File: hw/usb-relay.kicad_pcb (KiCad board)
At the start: 2 copper layers, 22 parts, among them IC1 ATTINY85-P, K1 RELAY_2RT, P1 USB_B, P2 CONN_02X03, Q1 BC548, U1 LM741

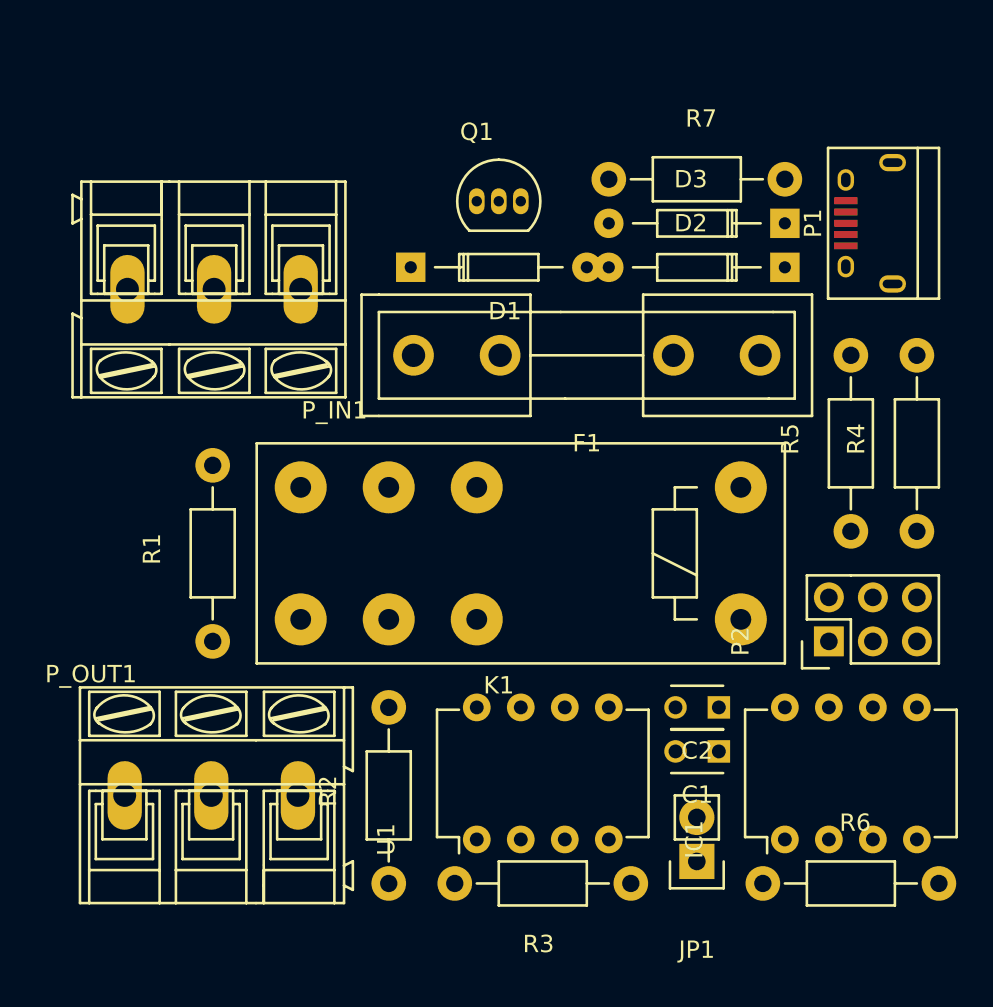
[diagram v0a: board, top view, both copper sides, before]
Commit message: Changes
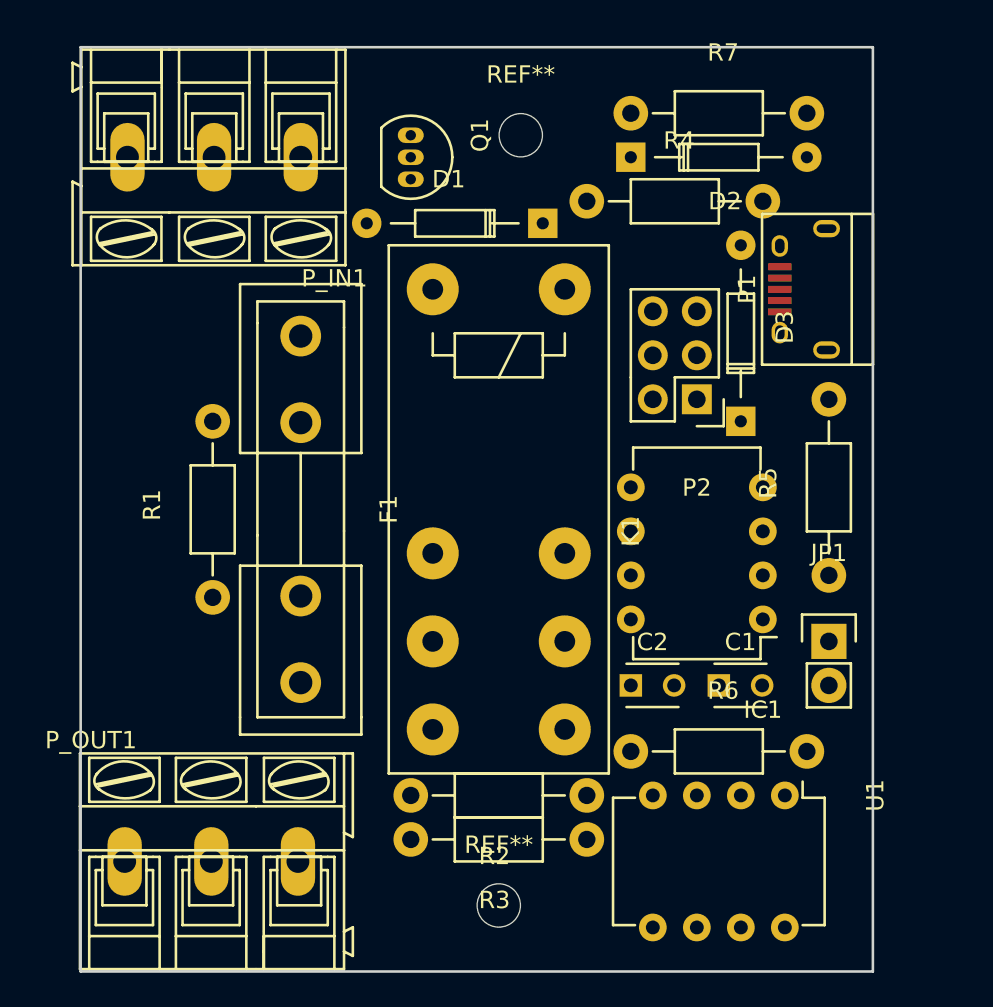
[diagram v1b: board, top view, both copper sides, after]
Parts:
- added REF**: MountingHole_2-5mm, Mounting_Holes:MountingHole_2-5mm, F.Cu at (76.2, 92.7)
- added REF**: MountingHole_2-5mm, Mounting_Holes:MountingHole_2-5mm, F.Cu at (74.9, 137.2)
- moved R4 26.9 mm to (80.0, 96.5), turned to 0 degrees
- moved K1 21.1 mm to (71.1, 101.6), turned to 270 degrees
- moved F1 18.8 mm to (63.5, 114.3), turned to 270 degrees
- moved U1 18.0 mm to (91.4, 130.8), turned to 270 degrees
- moved P2 15.9 mm to (86.4, 108.0), turned to 180 degrees
- moved JP1 14.8 mm to (94.0, 121.9), turned to 0 degrees
- moved IC1 12.8 mm to (90.2, 120.7), turned to 180 degrees
- moved R2 12.5 mm to (80.0, 130.8), turned to 180 degrees
- moved D3 11.7 mm to (88.9, 109.2), turned to 90 degrees
- moved D2 10.9 mm to (82.5, 94.0), turned to 0 degrees
- moved R6 10.8 mm to (82.5, 128.3)
- moved D1 8.03 mm to (77.5, 97.8), turned to 180 degrees
- moved P_IN1 7.62 mm to (63.5, 94.0)
- moved Q1 5.39 mm to (69.8, 92.7), turned to 270 degrees
- moved P1 5.39 mm to (92.7, 101.6)
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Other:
- board outline added: 45.7 x 53.3 mm
